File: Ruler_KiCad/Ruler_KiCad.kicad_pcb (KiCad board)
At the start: 2 copper layers, 155 x 30 mm, 24 parts

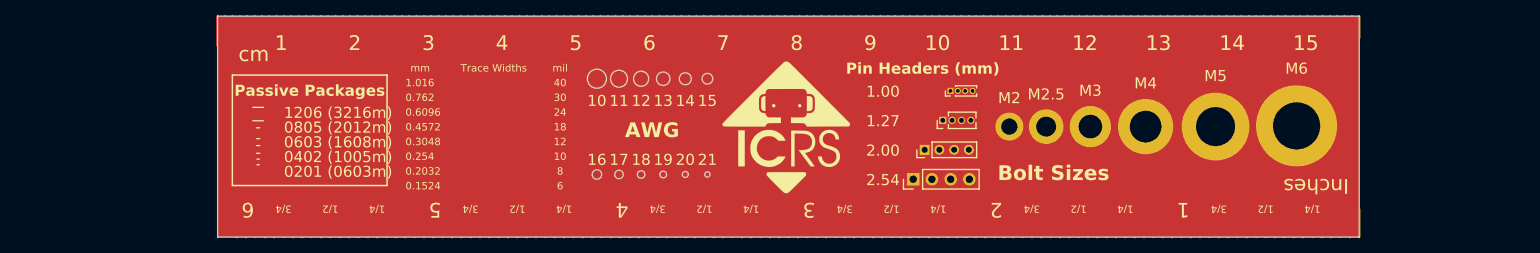
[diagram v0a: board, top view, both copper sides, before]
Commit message: New longer version
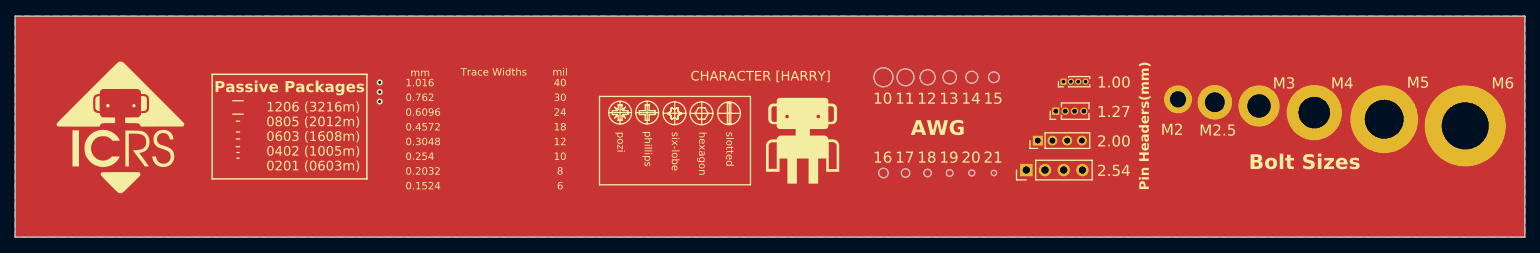
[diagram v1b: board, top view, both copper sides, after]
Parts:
- removed the REF** at (75.0, 85.0)
- removed the REF** at (230.0, 115.0)
- moved G*** 90.4 mm to (62.0, 100.0)
- moved G*** 39.4 mm to (118.1, 99.6)
- moved G*** 31.2 mm to (61.5, 97.7)
- moved REF** 23.2 mm to (205.4, 96.3)
- moved REF** 23.1 mm to (210.4, 96.7)
- moved REF** 23.1 mm to (216.4, 97.2)
- moved REF** 23.0 mm to (223.9, 98.1)
- moved REF** 22.9 mm to (233.4, 99.0)
- moved REF** 22.9 mm to (244.4, 99.9)
- moved REF** 16.3 mm to (90.2, 108.3)
- moved REF** 16.3 mm to (99.5, 108.0)
- moved REF** 16.3 mm to (82.8, 108.3)
- moved REF** 15.4 mm to (184.8, 105.9)
- moved REF** 15.4 mm to (189.8, 93.9)
- moved REF** 15.4 mm to (186.3, 101.9)
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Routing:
- net (no net): track 0.00 -> 105.0 mm
- net notvias: vias 0 -> 3
- added copper zone on B.Cu, net notvias
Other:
- board size 155 x 30 mm -> 205 x 30 mm
- board text added: "*hatched pour"
- board text added: "0.4"
- board text added: "0.6"
- board text added: "0.8"
- board text added: "1.6"
- board text added: "@icrobotics"
- board text added: "CHARACTER [HARRY]"
- board text added: "Designed by Laura and Ben 2026"
- board text added: "Layers"
- board text added: "Pin Headers(mm)"
- board text added: "Vocab"
- board text added: "copper"
- board text added: "curved"
- board text added: "hexagon"
- board text added: "mm"
- board text added: "pads"
- board text added: "phillips"
- board text added: "pozi"
- board text added: "sharp corner"
- board text added: "silkscreen"
- board text added: "six-lobe"
- board text added: "slotted"
- board text added: "solder mask"
- board text added: "substrate"
- board text added: "two bends"
- board text added: "vias"
- board text removed: "Designed by Ben Smith 2023"
- board text removed: "Inches"
- board text removed: "Pin Headers (mm)"
- board text removed: "cm"
